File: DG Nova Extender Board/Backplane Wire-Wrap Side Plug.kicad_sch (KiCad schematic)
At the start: 3 parts, among them J1 Port A, X1 A1, X3 A2

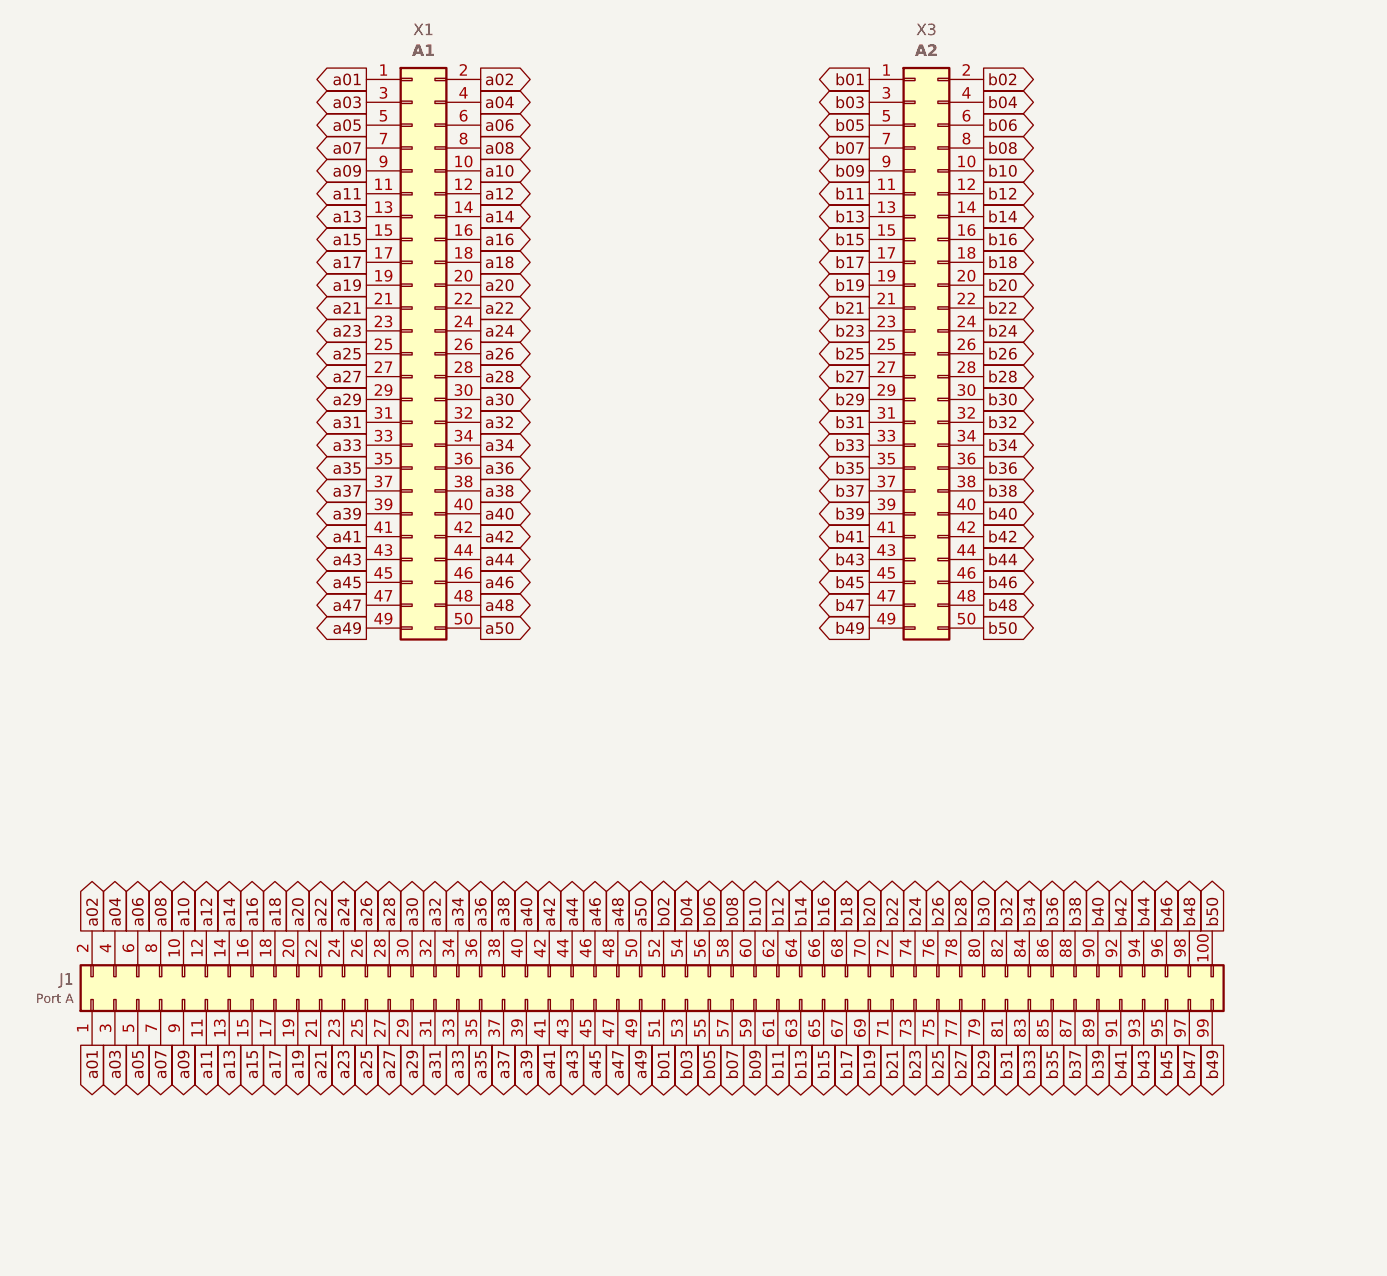
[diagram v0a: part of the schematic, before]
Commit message: Updates
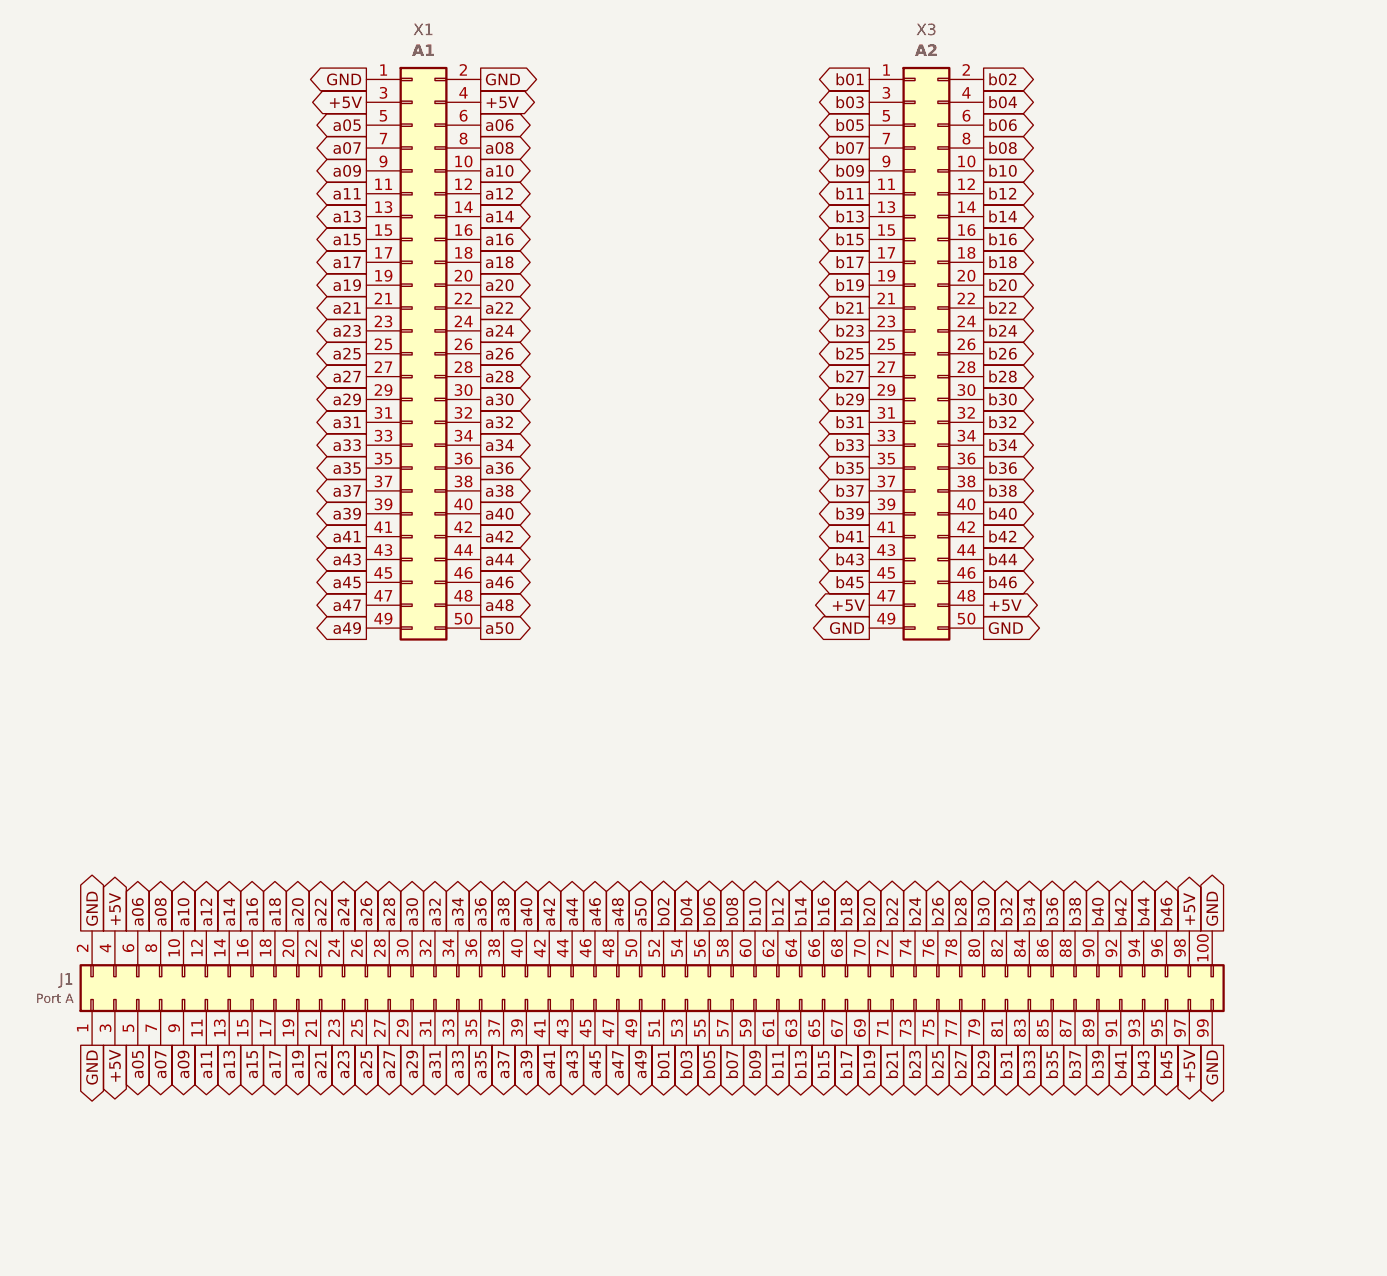
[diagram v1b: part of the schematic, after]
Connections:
- net a02 is gone; now on net GND: J1.2 (Pin_2), X1.2 (Pin_2)
- net a04 is gone; now on net +5V: J1.4 (Pin_4), X1.4 (Pin_4)
- net b47 is gone; now on net +5V: J1.97 (Pin_69), X3.47 (Pin_47)
- net b48 is gone; now on net +5V: J1.98 (Pin_98), X3.48 (Pin_48)
- net b49 is gone; now on net GND: J1.99 (Pin_99), X3.49 (Pin_49)
- net b50 is gone; now on net GND: J1.100 (Pin_100), X3.50 (Pin_50)
- net a01 renamed GND
- net a03 renamed +5V
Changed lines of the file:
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@@
     )
   )
-  (global_label "a02" (shape output) (at 71.12 32.385 0)
+  (global_label "GND" (shape output) (at 71.12 32.385 0)
     (effects (font (size 1.27 1.27)) (justify left))
     (property "Intersheetrefs" "${INTERSHEET_REFS}" (at 71.12 32.385 0)
@@
     )
   )
-  (global_label "b48" (shape output) (at 149.86 127 90)
+  (global_label "+5V" (shape output) (at 149.86 127 90)
     (effects (font (size 1.27 1.27)) (justify left))
     (property "Intersheetrefs" "${INTERSHEET_REFS}" (at 149.86 127 0)
@@
     )
   )
-  (global_label "a02" (shape output) (at 27.94 127 90)
+  (global_label "GND" (shape output) (at 27.94 127 90)
     (effects (font (size 1.27 1.27)) (justify left))
     (property "Intersheetrefs" "${INTERSHEET_REFS}" (at 27.94 127 0)
@@
     )
   )
-  (global_label "a04" (shape output) (at 30.48 127 90)
+  (global_label "+5V" (shape output) (at 30.48 127 90)
     (effects (font (size 1.27 1.27)) (justify left))
     (property "Intersheetrefs" "${INTERSHEET_REFS}" (at 30.48 127 0)
@@
     )
   )
-  (global_label "a01" (shape output) (at 58.42 32.385 180)
+  (global_label "GND" (shape output) (at 58.42 32.385 180)
     (effects (font (size 1.27 1.27)) (justify right))
     (property "Intersheetrefs" "${INTERSHEET_REFS}" (at 58.42 32.385 0)
@@
     )
   )
-  (global_label "a03" (shape output) (at 58.42 34.925 180)
+  (global_label "+5V" (shape output) (at 58.42 34.925 180)
     (effects (font (size 1.27 1.27)) (justify right))
     (property "Intersheetrefs" "${INTERSHEET_REFS}" (at 58.42 34.925 0)
@@
     )
   )
-  (global_label "a03" (shape output) (at 30.48 139.7 270)
+  (global_label "+5V" (shape output) (at 30.48 139.7 270)
     (effects (font (size 1.27 1.27)) (justify right))
     (property "Intersheetrefs" "${INTERSHEET_REFS}" (at 30.48 139.7 0)
@@
     )
   )
-  (global_label "b49" (shape output) (at 152.4 139.7 270)
+  (global_label "GND" (shape output) (at 152.4 139.7 270)
     (effects (font (size 1.27 1.27)) (justify right))
     (property "Intersheetrefs" "${INTERSHEET_REFS}" (at 152.4 139.7 0)
@@
     )
   )
-  (global_label "b49" (shape output) (at 114.3 93.345 180)
+  (global_label "GND" (shape output) (at 114.3 93.345 180)
     (effects (font (size 1.27 1.27)) (justify right))
     (property "Intersheetrefs" "${INTERSHEET_REFS}" (at 114.3 93.345 0)
@@
     )
   )
-  (global_label "b47" (shape output) (at 114.3 90.805 180)
+  (global_label "+5V" (shape output) (at 114.3 90.805 180)
     (effects (font (size 1.27 1.27)) (justify right))
     (property "Intersheetrefs" "${INTERSHEET_REFS}" (at 114.3 90.805 0)
@@
     )
   )
-  (global_label "a01" (shape output) (at 27.94 139.7 270)
+  (global_label "GND" (shape output) (at 27.94 139.7 270)
     (effects (font (size 1.27 1.27)) (justify right))
     (property "Intersheetrefs" "${INTERSHEET_REFS}" (at 27.94 139.7 0)
@@
     )
   )
-  (global_label "b48" (shape output) (at 127 90.805 0)
+  (global_label "+5V" (shape output) (at 127 90.805 0)
     (effects (font (size 1.27 1.27)) (justify left))
     (property "Intersheetrefs" "${INTERSHEET_REFS}" (at 127 90.805 0)
@@
     )
   )
-  (global_label "b47" (shape output) (at 149.86 139.7 270)
+  (global_label "+5V" (shape output) (at 149.86 139.7 270)
     (effects (font (size 1.27 1.27)) (justify right))
     (property "Intersheetrefs" "${INTERSHEET_REFS}" (at 149.86 139.7 0)
@@
     )
   )
-  (global_label "b50" (shape output) (at 127 93.345 0)
+  (global_label "GND" (shape output) (at 127 93.345 0)
     (effects (font (size 1.27 1.27)) (justify left))
     (property "Intersheetrefs" "${INTERSHEET_REFS}" (at 127 93.345 0)
@@
     )
   )
-  (global_label "a04" (shape output) (at 71.12 34.925 0)
+  (global_label "+5V" (shape output) (at 71.12 34.925 0)
     (effects (font (size 1.27 1.27)) (justify left))
     (property "Intersheetrefs" "${INTERSHEET_REFS}" (at 71.12 34.925 0)
@@
     )
   )
-  (global_label "b50" (shape output) (at 152.4 127 90)
+  (global_label "GND" (shape output) (at 152.4 127 90)
     (effects (font (size 1.27 1.27)) (justify left))
     (property "Intersheetrefs" "${INTERSHEET_REFS}" (at 152.4 127 0)
